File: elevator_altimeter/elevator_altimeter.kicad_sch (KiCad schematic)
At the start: 39 parts, among them J1 UART, J2 AVR-ICSP-TagConnect, J3 I2C, SW1 UserSW, U1 MPL3115A2, U2 NRF24L01_Breakout, U3 ATtiny1634-S, U4 MCP1711

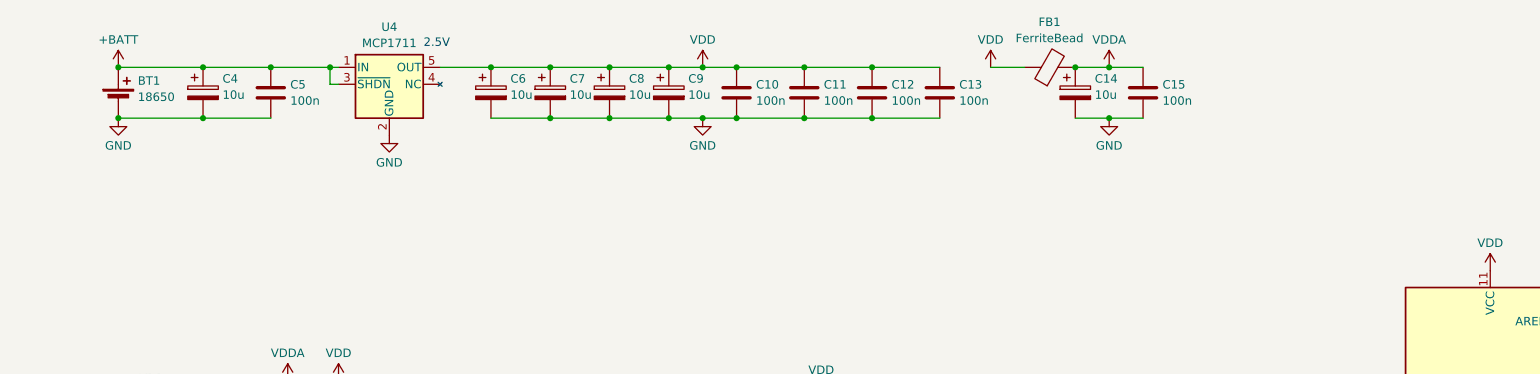
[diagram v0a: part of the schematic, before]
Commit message: a
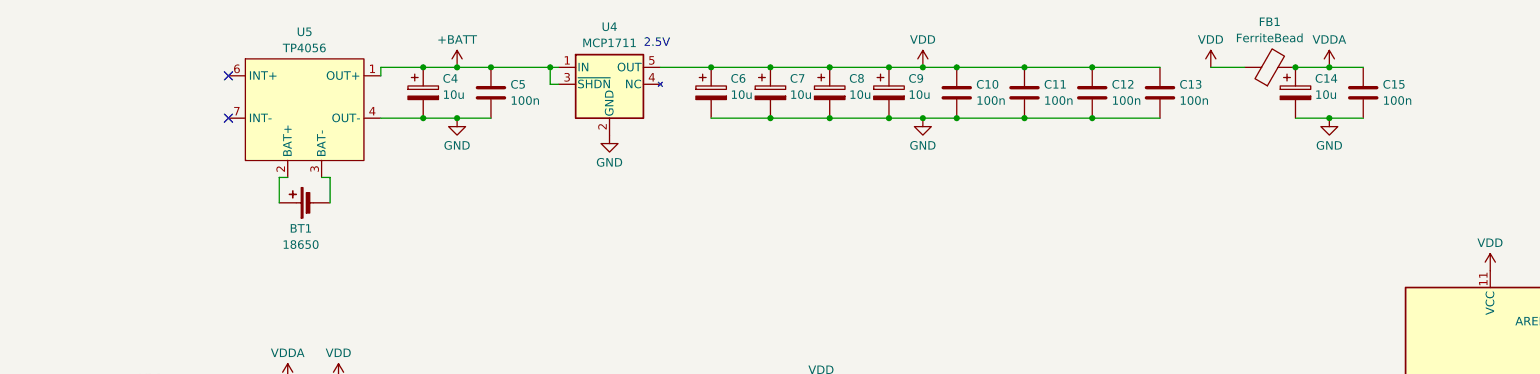
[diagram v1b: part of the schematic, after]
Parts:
- added U5: TP4056, footprints:TP4056_USB-C_module, symbol _MYLIBRARY:TP4056_USB-C_module
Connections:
- net +BATT: now also U5.1 (OUT+); no longer BT1.1 (+)
- net GND: now also U5.4 (OUT-); no longer BT1.2 (-)
- new net: BT1.1 (+), U5.2 (BAT+)
- new net: BT1.2 (-), U5.3 (BAT-)
- no-connect marks 4 -> 6
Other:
- moved on the sheet: BT1, C10, C11, C12, C13, C14, C15, C4, C5, C6, C7, C8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
